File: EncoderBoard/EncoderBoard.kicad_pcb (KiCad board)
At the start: 2 copper layers, 26.9 x 14.7 mm, 6 parts, among them P1 CONN_01X02, P2 CONN_01X02, U1 RPI-579N1

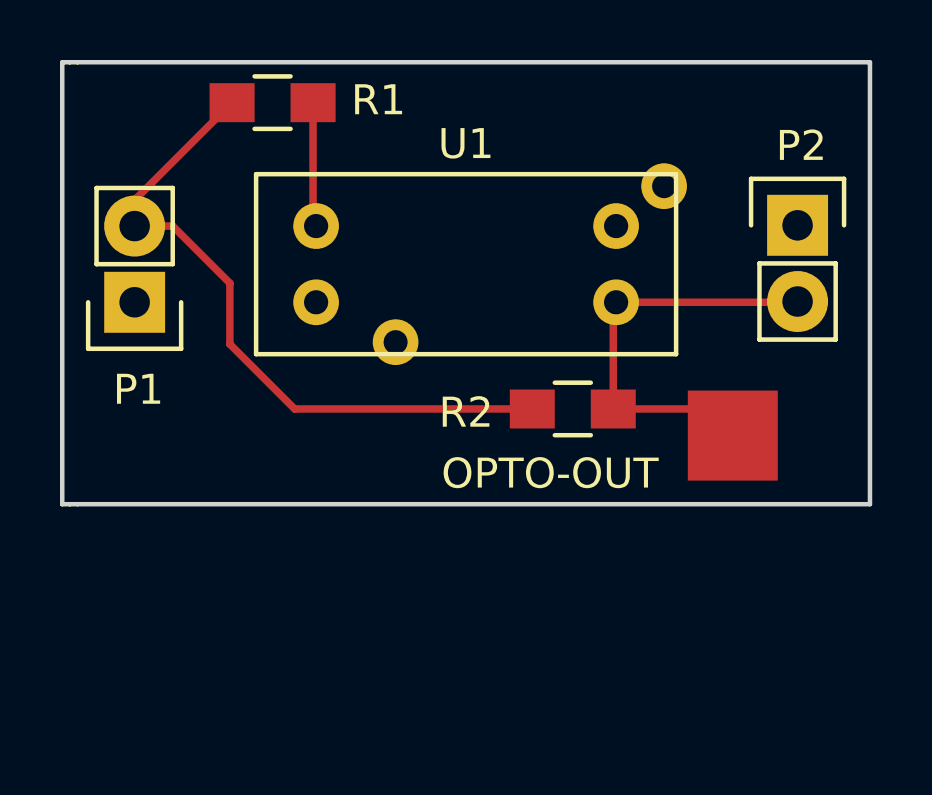
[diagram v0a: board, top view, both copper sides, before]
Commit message: generate gerbers
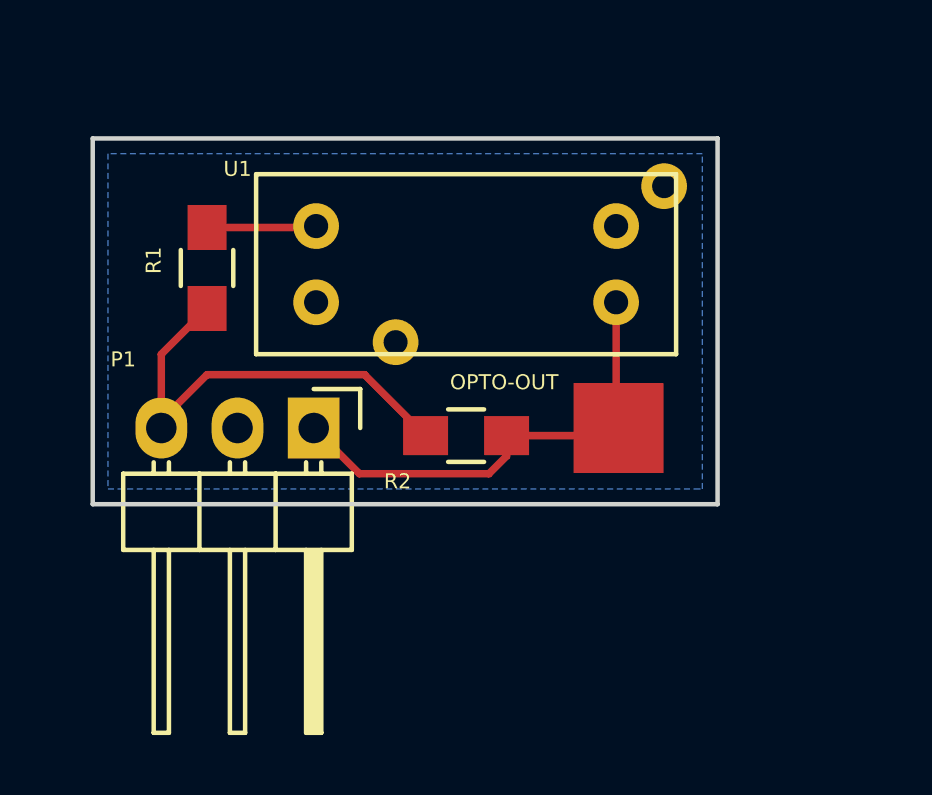
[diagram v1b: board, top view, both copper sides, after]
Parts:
- removed P2: CONN_01X02, Pin_Headers:Pin_Header_Straight_1x02
- P1: value CONN_01X02 -> CONN_01X03; footprint Pin_Headers:Pin_Header_Straight_1x02 -> Pin_Headers:Pin_Header_Angled_1x03
- moved P1 7.29 mm to (151.1, 115.3), turned to 270 degrees
- moved R1 5.93 mm to (147.6, 110.0), turned to 90 degrees
- moved W1 3.82 mm to (161.3, 115.3)
- moved R2 3.67 mm to (156.2, 115.6)
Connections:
- P1 pad 1: GND -> /Signal
- P1 pad 2: +5V -> GND
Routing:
- net +5V: track 22.4 -> 15.2 mm
- net /Signal: track 14.0 -> 16.0 mm
- net Net-(R1-Pad2): track 4.16 -> 3.66 mm
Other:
- board size 26.9 x 14.7 mm -> 20.8 x 12.2 mm
- board text added: "+5V"
- board text added: "Gnd"
- board text added: "GoGoGo Wheel Encoder Rev. 0"
- board text added: "Signal"

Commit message: adjusted soldermask and updated gerbers
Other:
- rule pad_to_mask_clearance: 0.2 -> 0.0762
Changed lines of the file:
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@@
     (pad_size 1.524 1.524)
     (pad_drill 0.762)
-    (pad_to_mask_clearance 0.2)
+    (pad_to_mask_clearance 0.0762)
+    (solder_mask_min_width 0.1016)
     (aux_axis_origin 0 0)
     (visible_elements FFFEFF7F)

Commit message: changed the pull up resistor to 3.3K
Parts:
- R2: value 1K -> 3.3K
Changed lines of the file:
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@@
     (links 8)
     (no_connects 0)
-    (area 143.688999 105.588999 164.667001 126.295801)
+    (area 143.688999 105.588999 164.667001 117.931001)
     (thickness 1.6)
     (drawings 9)
@@
       (effects (font (size 0.5 0.5) (thickness 0.1)))
     )
-    (fp_text value 1K (at 0 2.1) (layer F.Fab)
+    (fp_text value 3.3K (at 0 2.1) (layer F.Fab)
       (effects (font (size 0.5 0.5) (thickness 0.1)))
     )
